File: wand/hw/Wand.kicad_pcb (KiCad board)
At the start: 2 copper layers, 55 x 22.1 mm, 62 parts, among them J1 Conn_01x04, J2 Conn_01x08, J3 Conn_01x08, J4 Conn_01x04, J5 USB_C_Receptacle_PowerOnly_6P, M1 Vib, Q1 Si2301, Q2 Si2302, SW1 SW_SPST, SW2 Vib, U1 SPX3819M5-L-3-3, U2 STM32G030F6Px, U3 BMI270, U4 MMC5603NJ, U5 nRF24L01P, U6 LTC4054ES5-4.2, Y1 16MHz

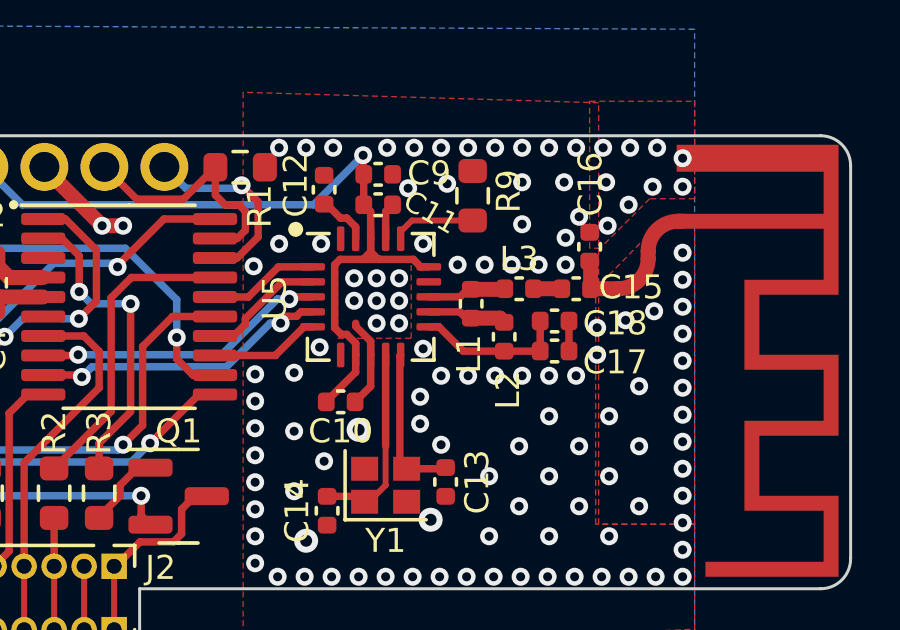
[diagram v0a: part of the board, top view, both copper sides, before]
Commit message: Revise central module hardware design
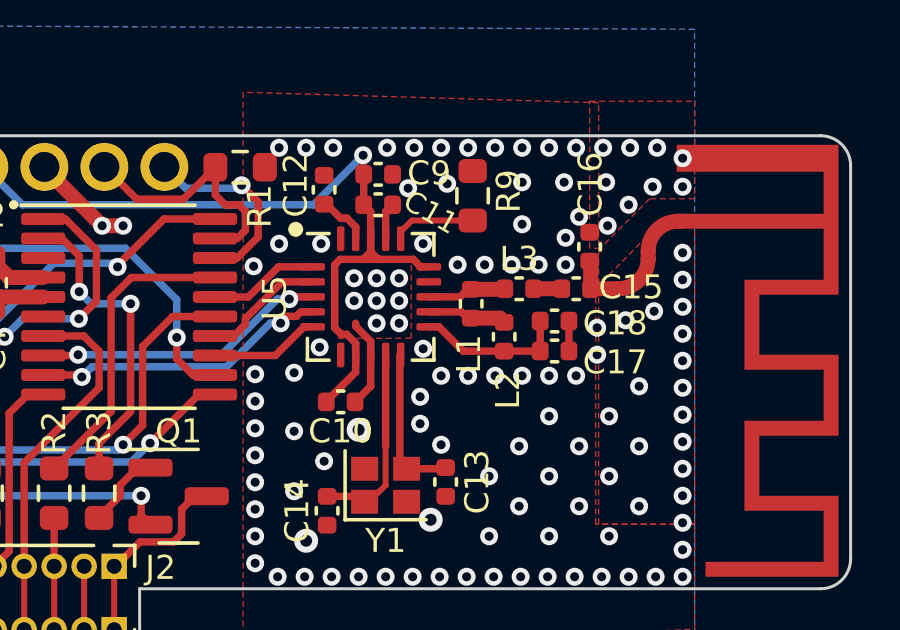
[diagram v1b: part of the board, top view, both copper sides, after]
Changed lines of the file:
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@@
   (segment (start 46.4 41.165) (end 46.4 42.9875) (width 0.2) (layer "B.Cu") (net 17))
   (segment (start 46.4 42.9875) (end 46.415 43.0025) (width 0.2) (layer "B.Cu") (net 17))
-  (segment (start 65.13 30.78) (end 64.92 30.57) (width 0.25) (layer "F.Cu") (net 18))
+  (segment (start 64.97 30.57) (end 63.889444 30.57) (width 0.25) (layer "F.Cu") (net 18))
+  (segment (start 65.18 30.78) (end 64.97 30.57) (width 0.25) (layer "F.Cu") (net 18))
   (segment (start 66.261944 30.78) (end 65.301944 30.78) (width 0.5) (layer "F.Cu") (net 18))
   (segment (start 66.401944 30.92) (end 66.261944 30.78) (width 0.5) (layer "F.Cu") (net 18))
-  (segment (start 64.92 30.57) (end 63.889444 30.57) (width 0.25) (layer "F.Cu") (net 18))
-  (segment (start 65.301944 30.78) (end 65.13 30.78) (width 0.25) (layer "F.Cu") (net 18))
+  (segment (start 65.301944 30.78) (end 65.18 30.78) (width 0.25) (layer "F.Cu") (net 18))
   (segment (start 65.301944 29.82) (end 66.401944 29.82) (width 0.5) (layer "F.Cu") (net 19))
   (segment (start 63.889444 30.07) (end 64.93 30.07) (width 0.25) (layer "F.Cu") (net 19))
@@
       1ae7fdbc-dc24-4dbc-8335-f601929143ab
       1ce4cfef-1acf-4f91-86d6-219b9e688972
-      2432a2b4-0238-4f92-a335-b42a5372838a
       260ba61f-c53f-48ba-97d8-69aef29b574b
       2cf0ce3f-27a7-4e31-857d-8bf2352fe25a
@@
       72d9d2f3-21e0-41fd-b522-1e49beed2d54
       77eeec9e-5196-4557-89b9-e1408de4fdab
-      7a6aa5ce-2b3f-4bca-8534-bc4ae8b043ef
       7f215527-fd74-4f46-9b45-7cf1f4273f97
       857b36a3-1857-4be7-9e62-4bf93613146f
@@
       aac73ff9-7c2a-4b0f-9ba8-7982bb59e4be
       aad41cf6-45bb-4206-82e5-5b1ebcf1a0d6
-      ae21d5ae-8dcd-4ffc-834b-fdd882701453
       b2763c0c-782e-4c52-9595-57bb1cbb5d06
       b5bc7fd7-ff48-4584-966c-9b43adf147ac
@@
       c4047f87-c49d-42de-815b-7f8c8990124c
       c65dcfb7-c88e-4f35-9369-7d2430eff168
-      c6faa4c7-a161-4178-9c94-144fc49306f4
-      c731ba39-48a5-466a-8692-24d08eaf518a
       c8ca79a4-6873-4674-a006-0a93bd8d45c7
       cafe9b43-99fd-42e9-9d24-f6b17f625389
-      cb68e2a9-ec28-4d02-927f-89dc716e6524
       cc473c23-7092-4962-b037-7fc8ef7d2fbd
       d1a13572-b16f-4866-a7e1-2e4a19a35828

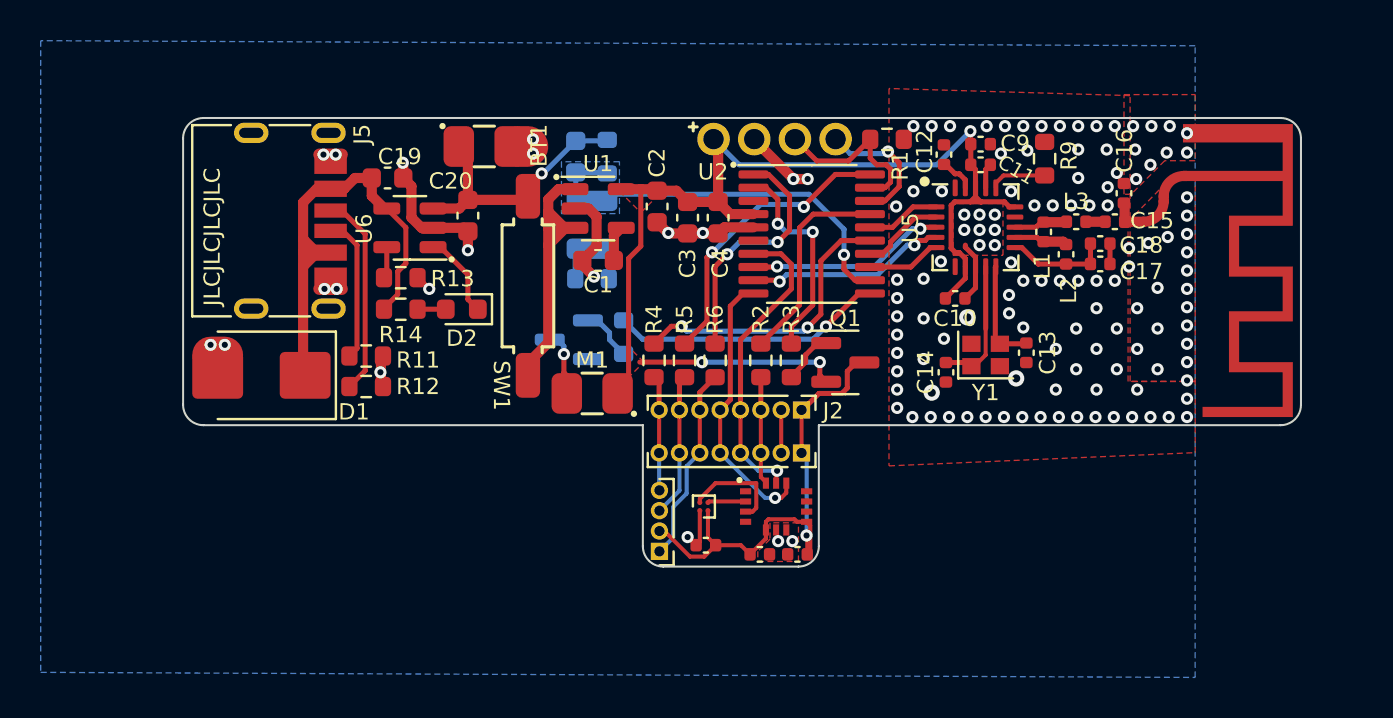
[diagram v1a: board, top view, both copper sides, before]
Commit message: Revise wand hardware design
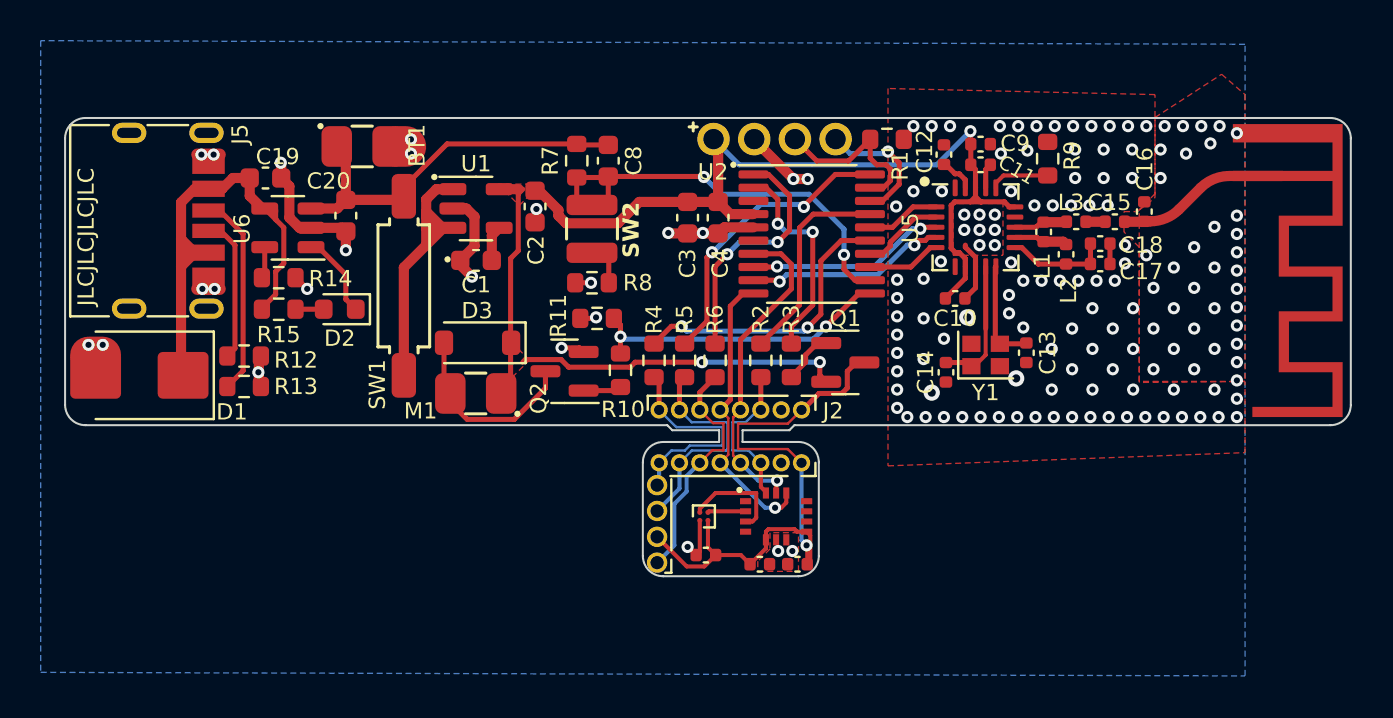
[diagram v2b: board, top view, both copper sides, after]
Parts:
- added D3: MBR0530, Diode_SMD:D_SOD-123, F.Cu at (37.5, 35.8)
- added R11: 100k, Resistor_SMD:R_0603_1608Metric, F.Cu at (43.4, 34.5)
- C8, Q2, R10, R7, R8, SW2: moved to F.Cu
- J4: footprint Connector_PinHeader_1.00mm:PinHeader_1x04_P1.00mm_Vertical -> Connector_PinHeader_1.27mm:PinHeader_1x04_P1.27mm_Vertical
- moved SW1 6.10 mm to (33.9, 33.0)
- moved BT1 6.00 mm to (31.8, 26.1)
- moved D2 6.00 mm to (30.7, 34.1)
- moved R14 6.00 mm to (27.7, 32.5)
- moved R15 6.00 mm to (27.7, 34.1)
- moved C1 6.00 mm to (37.4, 31.7)
- moved C2 6.00 mm to (40.3, 29.1)
- moved C20 6.00 mm to (31.0, 29.5)
- moved D1 6.00 mm to (20.9, 37.4)
- moved J5 6.00 mm to (21.4, 29.8)
- moved R12 6.00 mm to (26.0, 36.4)
- moved R13 6.00 mm to (26.0, 37.9)
- moved U1 6.00 mm to (37.4, 29.1)
- moved U6 6.00 mm to (28.1, 30.1)
- moved C19 6.00 mm to (27.1, 27.6)
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- renumbered R11 to R12, R12 to R13, R13 to R14, R14 to R15
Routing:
- net VDD: track 57.4 -> 69.4 mm
- net VDDSUB: track 24.7 -> 30.8 mm
- net Net-(D3-A): track 3.59 -> 9.55 mm, vias 1 -> 0
- net VBAT: track 13.0 -> 18.8 mm, vias 1 -> 0
- net LED_B: track 5.67 -> 10.7 mm
- net LED_G: track 7.07 -> 11.1 mm
- net Net-(AE1-Pad1): track 5.31 -> 8.45 mm
- net VIB_TRG: track 19.6 -> 22.4 mm, vias 1 -> 2
- net SPI2_MOSI: track 5.31 -> 7.88 mm
- net LED_R: track 9.70 -> 11.9 mm
- net MOTOR_G: track 13.4 -> 15.1 mm, vias 1 -> 2
- net BMI_CS: track 13.6 -> 14.4 mm
- net SPI2_SCK: track 15.2 -> 16.0 mm
- net Net-(Q2-G): track 2.64 -> 1.88 mm
- net GND: track 35.6 -> 36.2 mm, vias 137 -> 157
- removed copper zone on B.Cu, net VIB_TRG
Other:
- board size 55 x 22.1 mm -> 63.2 x 22.5 mm
- board text added: "Wand Rev. 3"
- board text removed: "Wand Rev. 2"
